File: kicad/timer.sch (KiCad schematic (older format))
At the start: 33 parts, among them IC1 STM8S003F3P, J1 PISK, J2 USB_OTG, J3 CONN_01X02, P1 kn1, P2 bat, P3 kn1, Q1 BC807-40, Q2 BC807-40, Q3 BC807-40, Q4 Q_NMOS_GSD, U1 TP4056

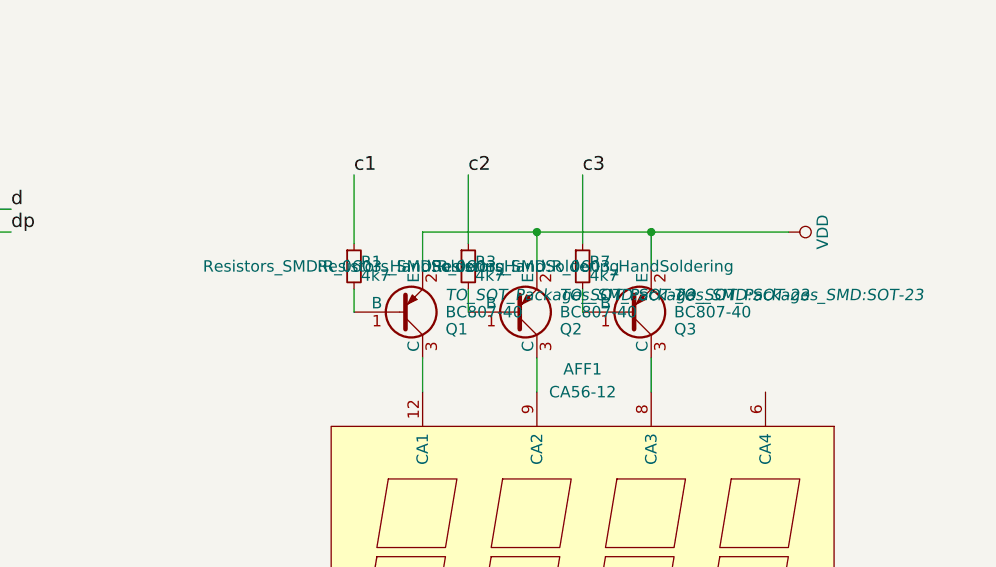
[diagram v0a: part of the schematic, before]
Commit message: start
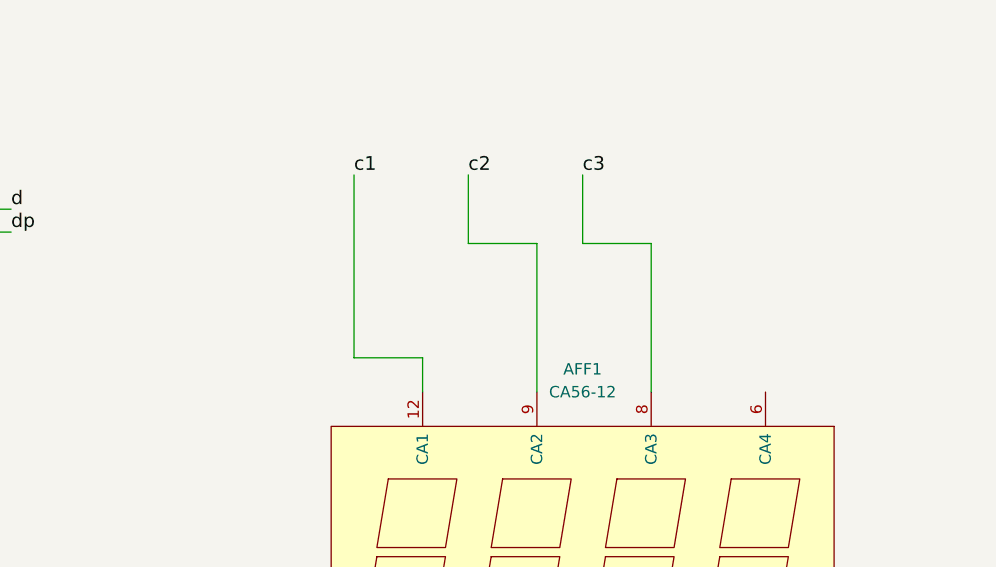
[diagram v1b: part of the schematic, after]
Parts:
- removed Q1, Q2, Q3: BC807-40, TO_SOT_Packages_SMD:SOT-23, symbol BC807-40
- removed R1, R3, R7: 4k7, Resistors_SMD:R_0603_HandSoldering, symbol R_Small
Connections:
- net c1: now also AFF1.12 (CA1)
- net c2: now also AFF1.9 (CA2)
- net c3: now also AFF1.8 (CA3)
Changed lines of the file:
@@
 LIBS:stm8
 LIBS:mylibkicad
-LIBS:kubik-cache
+LIBS:timer-cache
 EELAYER 25 0
 EELAYER END
@@
 Text Label 5600 2900 0    60   ~ 0
 dp
-$Comp
-L BC807-40 Q1
-U 1 1 58C44DC0
-P 7300 3250
-F 0 "Q1" H 7500 3325 50  0000 L CNN
-F 1 "BC807-40" H 7500 3250 50  0000 L CNN
-F 2 "TO_SOT_Packages_SMD:SOT-23" H 7500 3175 50  0000 L CIN
-F 3 "" H 7300 3250 50  0000 L CNN
-	1    7300 3250
-	1    0    0    1
-$EndComp
-$Comp
-L BC807-40 Q2
-U 1 1 58C45032
-P 7800 3250
-F 0 "Q2" H 8000 3325 50  0000 L CNN
-F 1 "BC807-40" H 8000 3250 50  0000 L CNN
-F 2 "TO_SOT_Packages_SMD:SOT-23" H 8000 3175 50  0000 L CIN
-F 3 "" H 7800 3250 50  0000 L CNN
-	1    7800 3250
-	1    0    0    1
-$EndComp
-$Comp
-L BC807-40 Q3
-U 1 1 58C450A4
-P 8300 3250
-F 0 "Q3" H 8500 3325 50  0000 L CNN
-F 1 "BC807-40" H 8500 3250 50  0000 L CNN
-F 2 "TO_SOT_Packages_SMD:SOT-23" H 8500 3175 50  0000 L CIN
-F 3 "" H 8300 3250 50  0000 L CNN
-	1    8300 3250
-	1    0    0    1
-$EndComp
-$Comp
-L VDD #PWR05
-U 1 1 58C454A6
-P 9000 2900
-F 0 "#PWR05" H 9000 2750 50  0001 C CNN
-F 1 "VDD" H 9000 3050 50  0000 C CNN
-F 2 "" H 9000 2900 50  0000 C CNN
-F 3 "" H 9000 2900 50  0000 C CNN
-	1    9000 2900
-	0    1    1    0
-$EndComp
-$Comp
-L R_Small R1
-U 1 1 58C4579E
-P 7100 3050
-F 0 "R1" H 7130 3070 50  0000 L CNN
-F 1 "4k7" H 7130 3010 50  0000 L CNN
-F 2 "Resistors_SMD:R_0603_HandSoldering" H 7100 3050 50  0000 C CNN
-F 3 "" H 7100 3050 50  0000 C CNN
-	1    7100 3050
-	1    0    0    -1
-$EndComp
-$Comp
-L R_Small R3
-U 1 1 58C4589D
-P 7600 3050
-F 0 "R3" H 7630 3070 50  0000 L CNN
-F 1 "4k7" H 7630 3010 50  0000 L CNN
-F 2 "Resistors_SMD:R_0603_HandSoldering" H 7600 3050 50  0000 C CNN
-F 3 "" H 7600 3050 50  0000 C CNN
-	1    7600 3050
-	1    0    0    -1
-$EndComp
-$Comp
-L R_Small R7
-U 1 1 58C45A71
-P 8100 3050
-F 0 "R7" H 8130 3070 50  0000 L CNN
-F 1 "4k7" H 8130 3010 50  0000 L CNN
-F 2 "Resistors_SMD:R_0603_HandSoldering" H 8100 3050 50  0000 C CNN
-F 3 "" H 8100 3050 50  0000 C CNN
-	1    8100 3050
-	1    0    0    -1
-$EndComp
 Text Label 7100 2650 0    60   ~ 0
 c1
@@
 	7400 3450 7400 3600
 Wire Wire Line
-	7900 3450 7900 3600
-Wire Wire Line
-	8400 3450 8400 3600
-Wire Wire Line
-	9000 2900 7400 2900
-Wire Wire Line
-	7400 2900 7400 3050
-Wire Wire Line
-	7900 3050 7900 2900
-Connection ~ 7900 2900
-Wire Wire Line
-	8400 3050 8400 2900
-Connection ~ 8400 2900
-Wire Wire Line
-	7100 3150 7100 3250
-Wire Wire Line
-	7600 3150 7600 3250
-Wire Wire Line
-	8100 3150 8100 3250
+	7900 2950 7900 3600
+Wire Wire Line
+	8400 2950 8400 3600
 Wire Wire Line
 	8100 2950 8100 2650
@@
 	7600 2950 7600 2650
 Wire Wire Line
-	7100 2650 7100 2950
+	7100 2650 7100 3450
 Wire Wire Line
 	2300 3200 2500 3200
@@
 Wire Wire Line
 	1400 4850 1550 4850
+Wire Wire Line
+	8100 2950 8400 2950
+Wire Wire Line
+	7600 2950 7900 2950
+Wire Wire Line
+	7100 3450 7400 3450
 $EndSCHEMATC

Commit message: start
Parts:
- AFF1: footprint mylibpcb:indicator_3cif -> myowndevice:indicator_3cif
- J2: footprint mylibpcb:usb5s -> myowndevice:usb5s
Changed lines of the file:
@@
 F 0 "AFF1" H 8100 5100 50  0000 C CNN
 F 1 "CA56-12" H 8100 5000 50  0000 C CNN
-F 2 "mylibpcb:indicator_3cif" H 7600 4300 50  0001 C CNN
+F 2 "myowndevice:indicator_3cif" H 7600 4300 50  0001 C CNN
 F 3 "" H 7600 4300 50  0000 C CNN
 	1    8100 4300
@@
 F 0 "J2" H 2500 5450 50  0000 L CNN
 F 1 "USB_OTG" H 2500 5350 50  0000 L CNN
-F 2 "mylibpcb:usb5s" H 2850 4950 50  0001 C CNN
+F 2 "myowndevice:usb5s" H 2850 4950 50  0001 C CNN
 F 3 "" H 2850 4950 50  0001 C CNN
 	1    2700 5000
